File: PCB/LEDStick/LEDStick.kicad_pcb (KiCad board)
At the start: 4 copper layers, 8.8 x 52.2 mm, 27 parts, among them J1 Conn_01x04_Pin

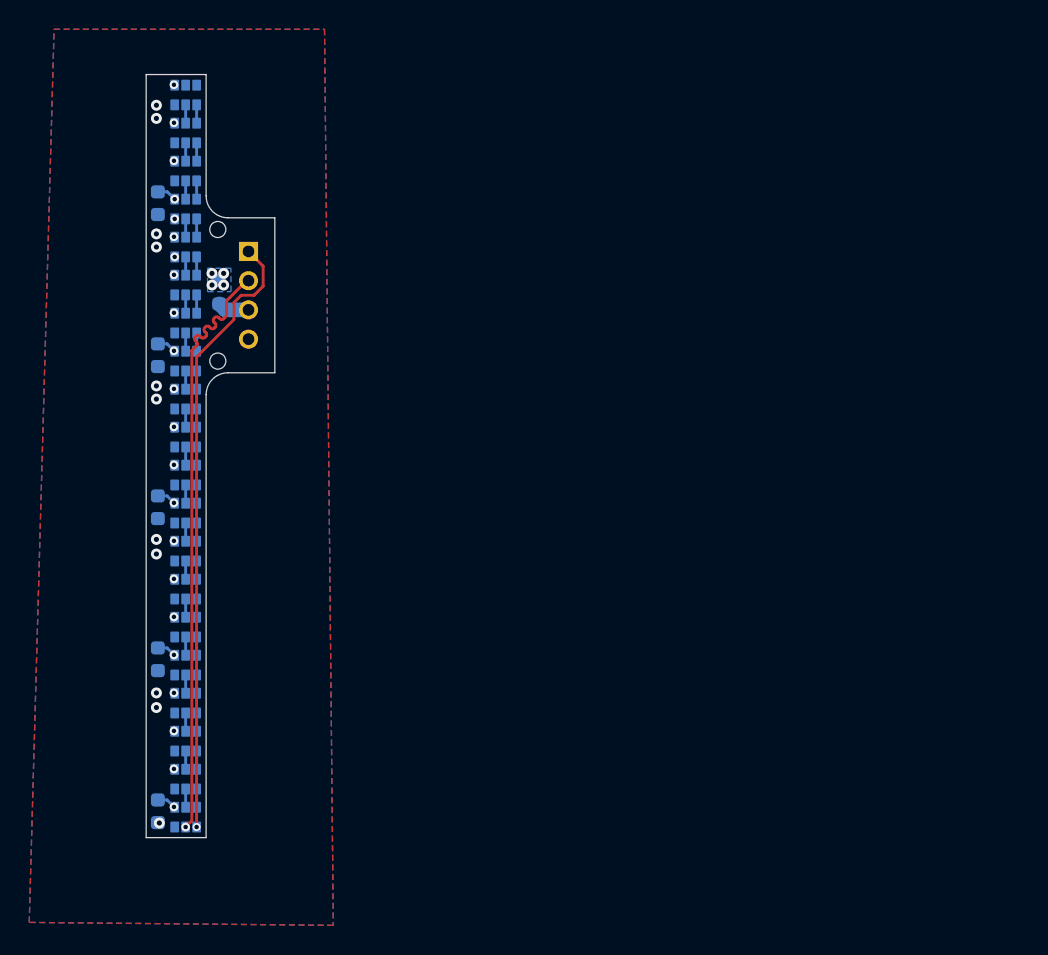
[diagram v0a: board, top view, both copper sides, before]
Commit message: boards ordered
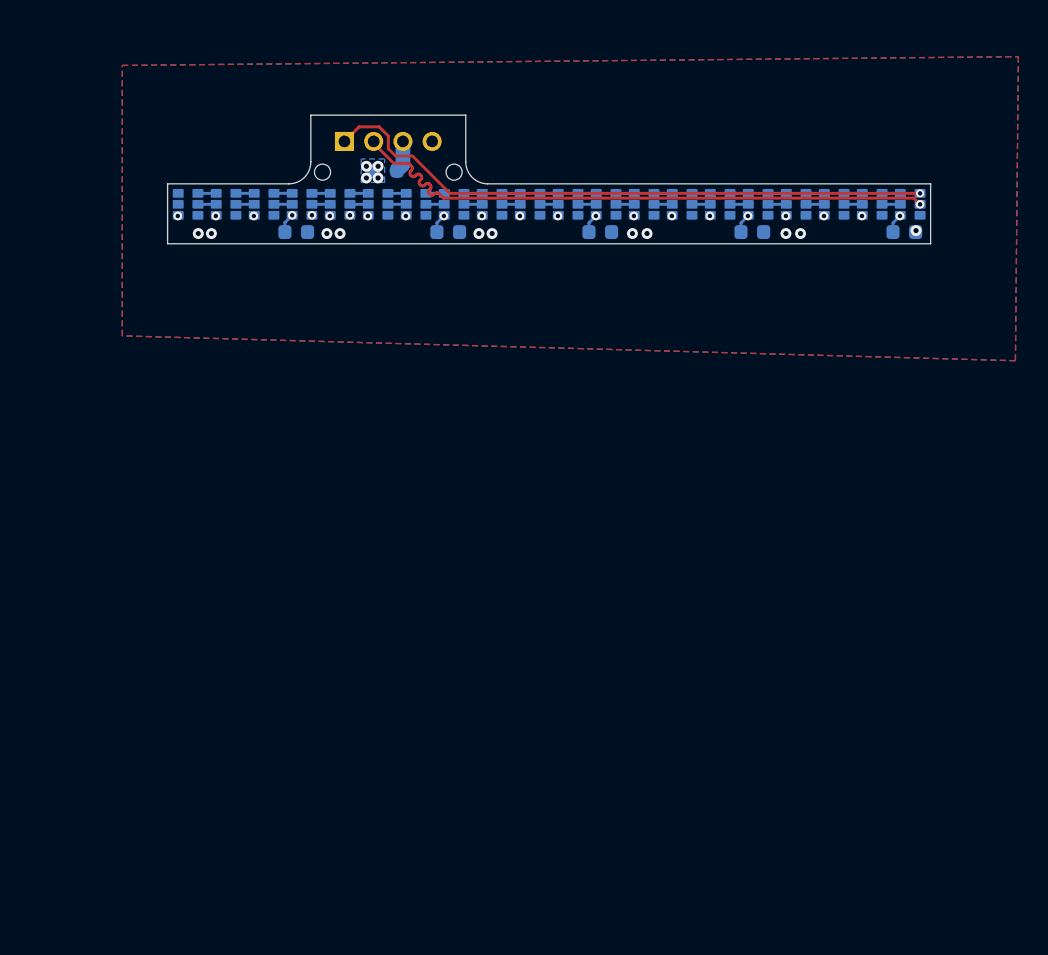
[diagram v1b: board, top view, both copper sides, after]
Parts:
- moved D1 64.9 mm to (77.3, 33.8), turned to 0 degrees
- moved C1 64.6 mm to (76.9, 35.7), turned to 0 degrees
- moved D2 61.3 mm to (74.7, 33.8), turned to 0 degrees
- moved D3 57.6 mm to (72.1, 33.8), turned to 0 degrees
- moved D4 53.9 mm to (69.5, 33.8), turned to 0 degrees
- moved D5 50.3 mm to (66.9, 33.8), turned to 0 degrees
- moved C2 50.1 mm to (66.5, 35.7), turned to 0 degrees
- moved D6 46.6 mm to (64.3, 33.8), turned to 0 degrees
- moved D7 43.0 mm to (61.7, 33.8), turned to 0 degrees
- moved D8 39.3 mm to (59.1, 33.8), turned to 0 degrees
- moved D9 35.7 mm to (56.5, 33.8), turned to 0 degrees
- moved C3 35.6 mm to (56.1, 35.7), turned to 0 degrees
- moved D10 32.1 mm to (53.9, 33.8), turned to 0 degrees
- moved D11 28.4 mm to (51.3, 33.8), turned to 0 degrees
- moved D12 24.8 mm to (48.7, 33.8), turned to 0 degrees
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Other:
- board size 8.8 x 52.2 mm -> 52.2 x 8.8 mm
